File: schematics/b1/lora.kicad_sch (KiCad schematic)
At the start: 4 parts, among them U4 Ai-Thinker-Ra-02

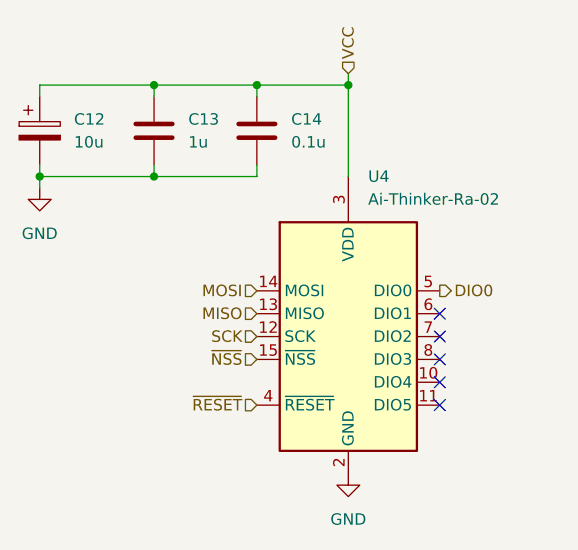
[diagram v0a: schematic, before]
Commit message: General schematic updates.
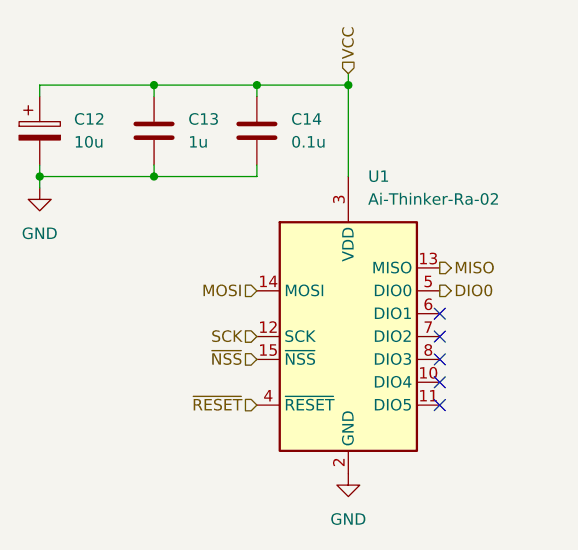
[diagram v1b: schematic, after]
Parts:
- renumbered U4 to U1
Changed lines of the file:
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@@
     (effects (font (size 1.27 1.27)) (justify right))
   )
-  (hierarchical_label "MISO" (shape input) (at 88.9 62.23 180) (fields_autoplaced)
-    (effects (font (size 1.27 1.27)) (justify right))
+  (hierarchical_label "MISO" (shape output) (at 109.22 57.15 0) (fields_autoplaced)
+    (effects (font (size 1.27 1.27)) (justify left))
   )
   (hierarchical_label "SCK" (shape input) (at 88.9 64.77 180) (fields_autoplaced)
@@
   (symbol (lib_id "power:GND") (at 99.06 80.01 0) (unit 1)
     (in_bom yes) (on_board yes) (dnp no) (fields_autoplaced)
-    (property "Reference" "#PWR022" (at 99.06 86.36 0)
+    (property "Reference" "#PWR02" (at 99.06 86.36 0)
       (effects (font (size 1.27 1.27)) hide)
     )
@@
       (project "b1"
         (path "/d6142fa5-2354-4512-9919-37616259c364/bca829a9-1cbe-4403-a4e4-7724b6c8becd"
-          (reference "#PWR022") (unit 1)
+          (reference "#PWR02") (unit 1)
         )
       )
@@
   (symbol (lib_id "power:GND") (at 64.77 48.26 0) (unit 1)
     (in_bom yes) (on_board yes) (dnp no) (fields_autoplaced)
-    (property "Reference" "#PWR023" (at 64.77 54.61 0)
+    (property "Reference" "#PWR01" (at 64.77 54.61 0)
       (effects (font (size 1.27 1.27)) hide)
     )
@@
       (project "b1"
         (path "/d6142fa5-2354-4512-9919-37616259c364/bca829a9-1cbe-4403-a4e4-7724b6c8becd"
-          (reference "#PWR023") (unit 1)
+          (reference "#PWR01") (unit 1)
         )
       )
@@
   (symbol (lib_id "RF_Module:Ai-Thinker-Ra-02") (at 99.06 64.77 0) (unit 1)
     (in_bom yes) (on_board yes) (dnp no) (fields_autoplaced)
-    (property "Reference" "U4" (at 101.2541 46.99 0)
+    (property "Reference" "U1" (at 101.2541 46.99 0)
       (effects (font (size 1.27 1.27)) (justify left))
     )
@@
       (project "b1"
         (path "/d6142fa5-2354-4512-9919-37616259c364/bca829a9-1cbe-4403-a4e4-7724b6c8becd"
-          (reference "U4") (unit 1)
+          (reference "U1") (unit 1)
         )
       )
